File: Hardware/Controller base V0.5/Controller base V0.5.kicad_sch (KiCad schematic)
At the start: 37 parts, among them J1 USB_C_Receptacle_USB2.0_16P, J2 Conn_01x05_Pin, J3 right face mod, J4 left face mod, J5 left sholder, J6 right sholder, SW1 SW_Push, SW2 SW_Push, SW3 SW_Push, SW4 SW_Push, U1 AZ1117CH-3.3TRG1, U2 ESP32-S3-WROOM-1U-N4

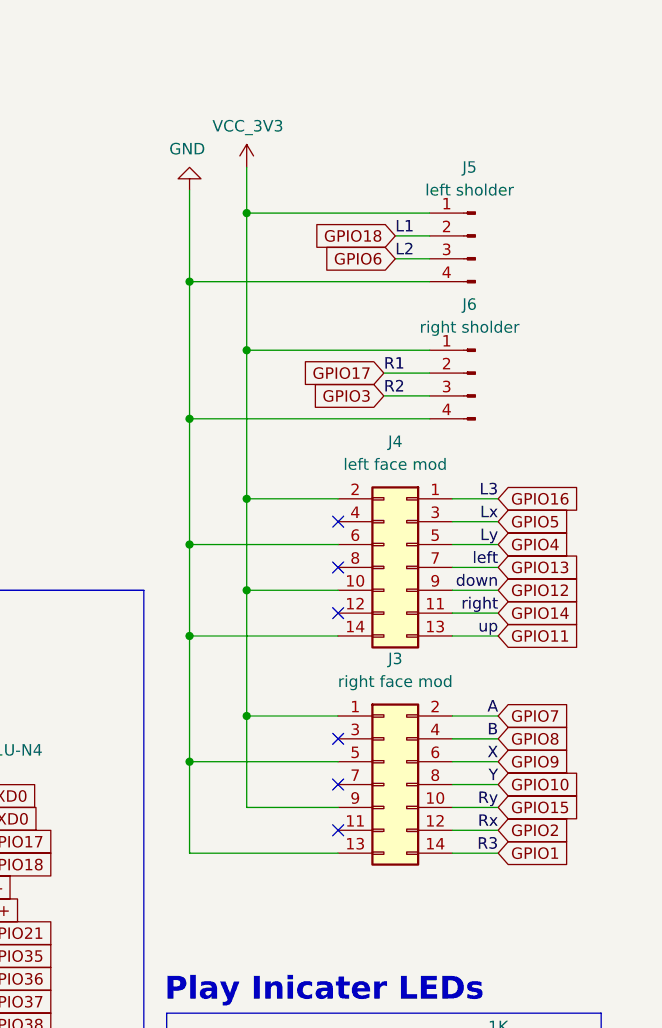
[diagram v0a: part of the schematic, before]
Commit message: update
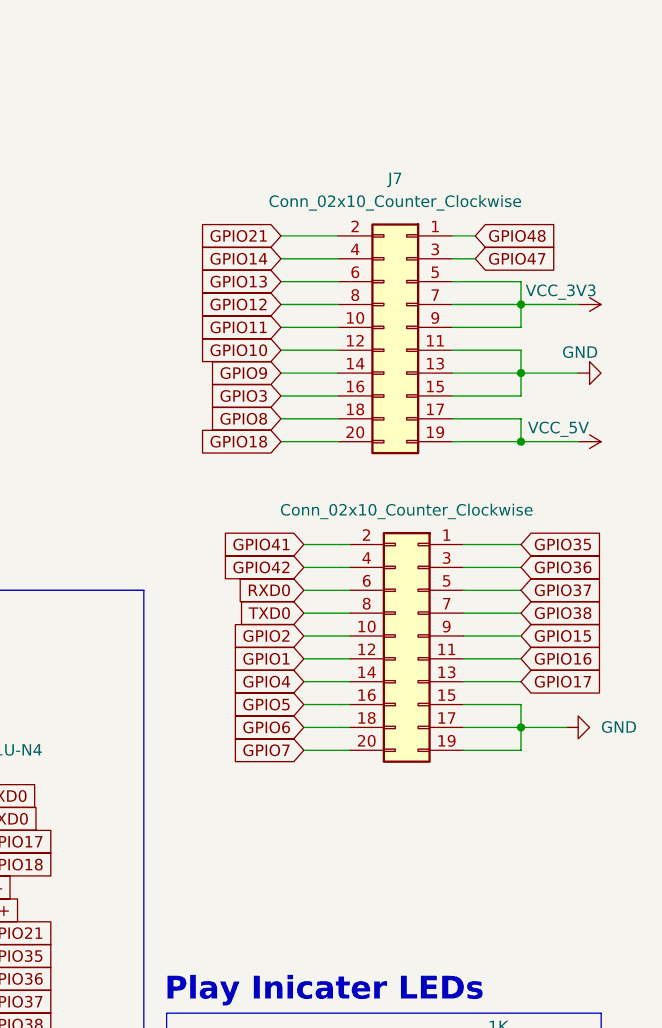
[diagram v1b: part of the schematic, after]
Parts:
- removed J3: right face mod, Connector_PinHeader_1.27mm:PinHeader_2x07_P1.27mm_Vertical, symbol Connector_Generic:Conn_02x07_Odd_Even
- removed J4: left face mod, Connector_PinHeader_1.27mm:PinHeader_2x07_P1.27mm_Vertical, symbol Connector_Generic:Conn_02x07_Odd_Even
- removed J5: left sholder, Connector_PinHeader_1.27mm:PinHeader_1x04_P1.27mm_Vertical, symbol Library:Conn_01x04_Pin
- removed J6: right sholder, Connector_PinHeader_1.27mm:PinHeader_1x04_P1.27mm_Vertical, symbol Library:Conn_01x04_Pin
- added J7, J8: Conn_02x10_Counter_Clockwise, Connector_Hirose_DF40:Hirose_DF40C-20DS-0.4V_2x10_P0.4mm, symbol Connector_Generic:Conn_02x10_Odd_Even
- C1, C2, C4, C5, C6, C7, C8: footprint Capacitor_SMD:C_0805_2012Metric_Pad1.18x1.45mm_HandSolder -> Capacitor_SMD:C_0603_1608Metric_Pad1.08x0.95mm_HandSolder
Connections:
- net GND: now also J7.11 (Pin_11), J7.13 (Pin_13), J7.15 (Pin_15), J8.15 (Pin_15), J8.17 (Pin_17), J8.19 (Pin_19)
- net GPIO1: now also J8.12 (Pin_12); no longer U2.8 (IO15)
- net GPIO10: now also J7.12 (Pin_12)
- net GPIO11: now also J7.10 (Pin_10)
- net GPIO12: now also J7.8 (Pin_8)
- net GPIO13: now also J7.6 (Pin_6)
- net GPIO14: now also J7.4 (Pin_4)
- net GPIO16: now also J8.11 (Pin_11)
- net GPIO17: now also J8.13 (Pin_13)
- net GPIO18: now also J7.20 (Pin_20)
- net GPIO2: now also J8.10 (Pin_10)
- net GPIO21: now also J7.2 (Pin_2)
- net GPIO3: now also J7.16 (Pin_16)
- net GPIO35: now also J8.1 (Pin_1)
- net GPIO36: now also J8.3 (Pin_3)
- net GPIO37: now also J8.5 (Pin_5)
- net GPIO38: now also J8.7 (Pin_7)
- net GPIO4: now also J8.14 (Pin_14)
- net GPIO41: now also J8.2 (Pin_2)
- net GPIO42: now also J8.4 (Pin_4)
- net GPIO47: now also J7.3 (Pin_3)
- net GPIO48: now also J7.1 (Pin_1)
- net GPIO5: now also J8.16 (Pin_16)
- net GPIO6: now also J8.18 (Pin_18)
- net GPIO7: now also J8.20 (Pin_20)
- net GPIO8: now also J7.18 (Pin_18)
- net GPIO9: now also J7.14 (Pin_14)
- net RXD0: now also J8.6 (Pin_6)
- net TXD0: now also J8.8 (Pin_8)
- net VCC_3V3: now also J7.5 (Pin_5), J7.7 (Pin_7), J7.9 (Pin_9)
- net VCC_5V: now also J7.17 (Pin_17), J7.19 (Pin_19)
- new net GPIO15: J8.9 (Pin_9), U2.8 (IO15)
- no-connect marks 12 -> 6
